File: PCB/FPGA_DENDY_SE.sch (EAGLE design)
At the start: 139 parts, among them CN1 DENDY60PINSLOT, J1 NTSC/PAL, J2 DENDY, Q1 14.318 MHz, Q2 17.734 MHz, U1 EP1C3T100C8N, U10 OPA2134U, U11 SN74LVC2G34DBVR, U12 THS7314DR, U13 74LS373WMSO20, U14 SN74LVC1G125DBVR, U15 74LVC1G04GV, U16 SN74LVC1G3157, U2 EPCS4, U3 SN74LVC8T245, U4 SN74LVC8T245, U5 SN74LVC1G240DBVR, U6 SN74LVC1G240DBVR, U7 SN74LVC1G240DBVR, U8 SN74LVC1G240DBVR, X1 057-010-1

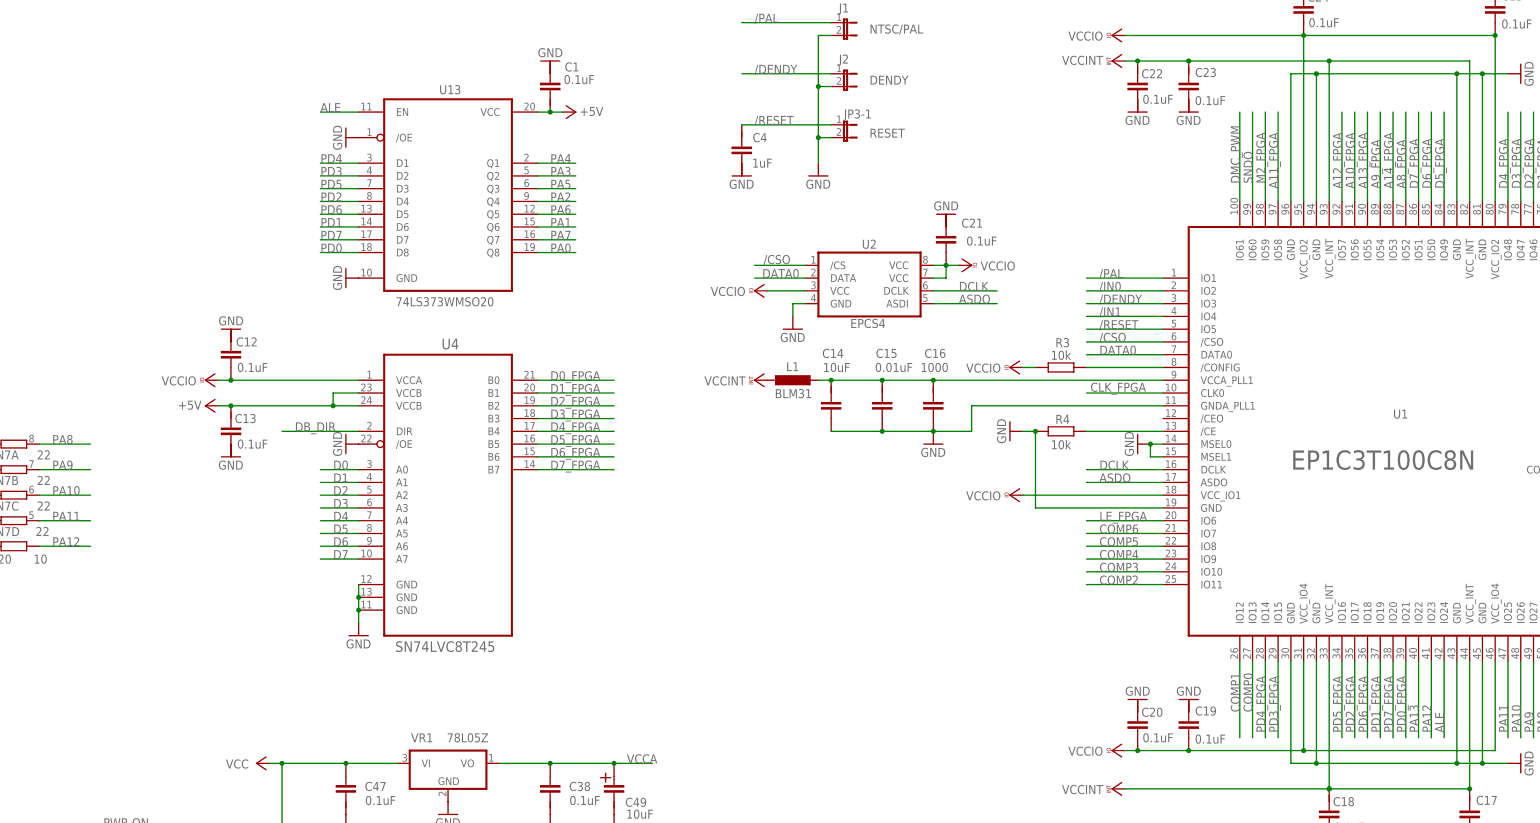
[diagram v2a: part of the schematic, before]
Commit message: Add files via upload
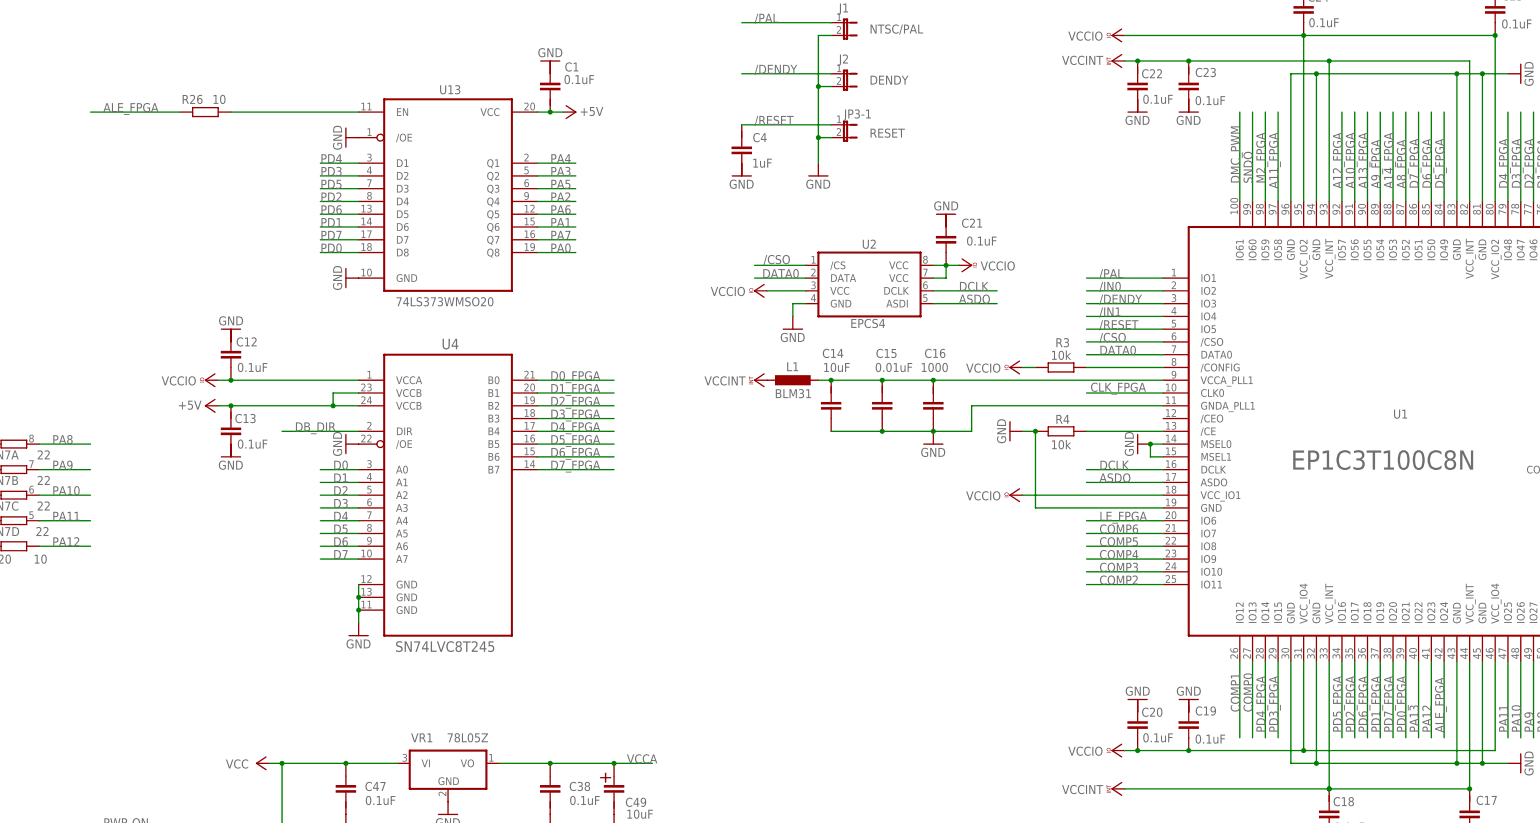
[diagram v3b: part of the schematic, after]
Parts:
- added R26: 10, rcl:R-EU_R0805
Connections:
- removed net ALE: U1.IO24, U13.EN
- new net ALE_FPGA: R26.1, U1.IO24
- new net N$6: R26.2, U13.EN
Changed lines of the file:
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@@
 <setting verticaltext="up"/>
 </settings>
-<grid distance="0.1" unitdist="inch" unit="inch" style="lines" multiple="1" display="no" altdistance="0.01" altunitdist="inch" altunit="inch"/>
+<grid distance="0.1" unitdist="inch" unit="inch" style="lines" multiple="1" display="yes" altdistance="0.01" altunitdist="inch" altunit="inch"/>
 <layers>
-<layer number="1" name="Top" color="4" fill="1" visible="yes" active="no"/>
-<layer number="2" name="Route2" color="16" fill="1" visible="yes" active="no"/>
-<layer number="3" name="Route3" color="17" fill="1" visible="yes" active="no"/>
-<layer number="4" name="Route4" color="18" fill="1" visible="yes" active="no"/>
-<layer number="5" name="Route5" color="19" fill="1" visible="yes" active="no"/>
-<layer number="6" name="Route6" color="25" fill="1" visible="yes" active="no"/>
-<layer number="7" name="Route7" color="26" fill="1" visible="yes" active="no"/>
-<layer number="8" name="Route8" color="27" fill="1" visible="yes" active="no"/>
-<layer number="9" name="Route9" color="28" fill="1" visible="yes" active="no"/>
-<layer number="10" name="Route10" color="29" fill="1" visible="yes" active="no"/>
-<layer number="11" name="Route11" color="30" fill="1" visible="yes" active="no"/>
-<layer number="12" name="Route12" color="20" fill="1" visible="yes" active="no"/>
-<layer number="13" name="Route13" color="21" fill="1" visible="yes" active="no"/>
-<layer number="14" name="Route14" color="22" fill="1" visible="yes" active="no"/>
-<layer number="15" name="Route15" color="23" fill="1" visible="yes" active="no"/>
-<layer number="16" name="Bottom" color="1" fill="1" visible="yes" active="no"/>
-<layer number="17" name="Pads" color="2" fill="1" visible="yes" active="no"/>
-<layer number="18" name="Vias" color="2" fill="1" visible="yes" active="no"/>
-<layer number="19" name="Unrouted" color="6" fill="1" visible="yes" active="no"/>
-<layer number="20" name="Dimension" color="15" fill="1" visible="yes" active="no"/>
-<layer number="21" name="tPlace" color="7" fill="1" visible="yes" active="no"/>
-<layer number="22" name="bPlace" color="7" fill="1" visible="yes" active="no"/>
-<layer number="23" name="tOrigins" color="15" fill="1" visible="yes" active="no"/>
-<layer number="24" name="bOrigins" color="15" fill="1" visible="yes" active="no"/>
-<layer number="25" name="tNames" color="7" fill="1" visible="yes" active="no"/>
-<layer number="26" name="bNames" color="7" fill="1" visible="yes" active="no"/>
-<layer number="27" name="tValues" color="7" fill="1" visible="yes" active="no"/>
-<layer number="28" name="bValues" color="7" fill="1" visible="yes" active="no"/>
+<layer number="1" name="Top" color="4" fill="1" visible="no" active="no"/>
+<layer number="2" name="Route2" color="16" fill="1" visible="no" active="no"/>
+<layer number="3" name="Route3" color="17" fill="1" visible="no" active="no"/>
+<layer number="4" name="Route4" color="18" fill="1" visible="no" active="no"/>
+<layer number="5" name="Route5" color="19" fill="1" visible="no" active="no"/>
+<layer number="6" name="Route6" color="25" fill="1" visible="no" active="no"/>
+<layer number="7" name="Route7" color="26" fill="1" visible="no" active="no"/>
+<layer number="8" name="Route8" color="27" fill="1" visible="no" active="no"/>
+<layer number="9" name="Route9" color="28" fill="1" visible="no" active="no"/>
+<layer number="10" name="Route10" color="29" fill="1" visible="no" active="no"/>
+<layer number="11" name="Route11" color="30" fill="1" visible="no" active="no"/>
+<layer number="12" name="Route12" color="20" fill="1" visible="no" active="no"/>
+<layer number="13" name="Route13" color="21" fill="1" visible="no" active="no"/>
+<layer number="14" name="Route14" color="22" fill="1" visible="no" active="no"/>
+<layer number="15" name="Route15" color="23" fill="1" visible="no" active="no"/>
+<layer number="16" name="Bottom" color="1" fill="1" visible="no" active="no"/>
+<layer number="17" name="Pads" color="2" fill="1" visible="no" active="no"/>
+<layer number="18" name="Vias" color="2" fill="1" visible="no" active="no"/>
+<layer number="19" name="Unrouted" color="6" fill="1" visible="no" active="no"/>
+<layer number="20" name="Dimension" color="15" fill="1" visible="no" active="no"/>
+<layer number="21" name="tPlace" color="7" fill="1" visible="no" active="no"/>
+<layer number="22" name="bPlace" color="7" fill="1" visible="no" active="no"/>
+<layer number="23" name="tOrigins" color="15" fill="1" visible="no" active="no"/>
+<layer number="24" name="bOrigins" color="15" fill="1" visible="no" active="no"/>
+<layer number="25" name="tNames" color="7" fill="1" visible="no" active="no"/>
+<layer number="26" name="bNames" color="7" fill="1" visible="no" active="no"/>
+<layer number="27" name="tValues" color="7" fill="1" visible="no" active="no"/>
+<layer number="28" name="bValues" color="7" fill="1" visible="no" active="no"/>
 <layer number="29" name="tStop" color="7" fill="3" visible="no" active="no"/>
 <layer number="30" name="bStop" color="7" fill="6" visible="no" active="no"/>
@@
 <layer number="35" name="tGlue" color="7" fill="4" visible="no" active="no"/>
 <layer number="36" name="bGlue" color="7" fill="5" visible="no" active="no"/>
-<layer number="37" name="tTest" color="7" fill="1" visible="yes" active="no"/>
-<layer number="38" name="bTest" color="7" fill="1" visible="yes" active="no"/>
+<layer number="37" name="tTest" color="7" fill="1" visible="no" active="no"/>
+<layer number="38" name="bTest" color="7" fill="1" visible="no" active="no"/>
 <layer number="39" name="tKeepout" color="4" fill="11" visible="no" active="no"/>
 <layer number="40" name="bKeepout" color="1" fill="11" visible="no" active="no"/>
@@
 <layer number="44" name="Drills" color="7" fill="1" visible="no" active="no"/>
 <layer number="45" name="Holes" color="7" fill="1" visible="no" active="no"/>
-<layer number="46" name="Milling" color="3" fill="1" visible="yes" active="no"/>
-<layer number="47" name="Measures" color="7" fill="1" visible="yes" active="no"/>
-<layer number="48" name="Document" color="7" fill="1" visible="yes" active="no"/>
-<layer number="49" name="Reference" color="7" fill="1" visible="yes" active="no"/>
-<layer number="50" name="dxf" color="7" fill="1" visible="yes" active="no"/>
-<layer number="51" name="tDocu" color="7" fill="1" visible="yes" active="no"/>
-<layer number="52" name="bDocu" color="7" fill="1" visible="yes" active="no"/>
-<layer number="56" name="wert" color="7" fill="1" visible="yes" active="no"/>
+<layer number="46" name="Milling" color="3" fill="1" visible="no" active="no"/>
+<layer number="47" name="Measures" color="7" fill="1" visible="no" active="no"/>
+<layer number="48" name="Document" color="7" fill="1" visible="no" active="no"/>
+<layer number="49" name="Reference" color="7" fill="1" visible="no" active="no"/>
+<layer number="50" name="dxf" color="7" fill="1" visible="no" active="no"/>
+<layer number="51" name="tDocu" color="7" fill="1" visible="no" active="no"/>
+<layer number="52" name="bDocu" color="7" fill="1" visible="no" active="no"/>
+<layer number="56" name="wert" color="7" fill="1" visible="no" active="no"/>
 <layer number="88" name="SimResults" color="9" fill="1" visible="yes" active="yes"/>
 <layer number="89" name="SimProbes" color="9" fill="1" visible="yes" active="yes"/>
@@
 <part name="GND81" library="supply1" library_urn="urn:adsk.eagle:library:371" deviceset="GND" device=""/>
 <part name="VCC15" library="supply1" library_urn="urn:adsk.eagle:library:371" deviceset="VCCIO" device=""/>
+<part name="R26" library="rcl" library_urn="urn:adsk.eagle:library:334" deviceset="R-EU_" device="R0805" package3d_urn="urn:adsk.eagle:package:23553/2" value="10"/>
 </parts>
 <sheets>
@@
 <attribute name="VALUE" x="29.718" y="158.242" size="1.778" layer="96" rot="MR180"/>
 </instance>
+<instance part="R26" gate="G$1" x="-236.22" y="60.96" smashed="yes">
+<attribute name="NAME" x="-236.648" y="64.3626" size="1.778" layer="95" rot="R180"/>
+<attribute name="VALUE" x="-232.068" y="64.368" size="1.778" layer="96" rot="R180"/>
+</instance>
 </instances>
 <busses>
@@
 </segment>
 </net>
-<net name="ALE" class="0">
-<segment>
-<wire x1="10.16" y1="-48.26" x2="10.16" y2="-63.5" width="0.1524" layer="91"/>
-<label x="10.16" y="-62.484" size="1.778" layer="95" rot="R90"/>
-<pinref part="U1" gate="G$1" pin="IO24"/>
-</segment>
-<segment>
-<wire x1="-205.74" y1="60.96" x2="-213.36" y2="60.96" width="0.1524" layer="91"/>
-<label x="-213.36" y="60.96" size="1.778" layer="95"/>
-<pinref part="U13" gate="G$1" pin="EN"/>
-</segment>
-</net>
 <net name="N$17" class="0">
 <segment>
@@
 </segment>
 </net>
+<net name="ALE_FPGA" class="0">
+<segment>
+<wire x1="10.16" y1="-48.26" x2="10.16" y2="-63.5" width="0.1524" layer="91"/>
+<label x="10.16" y="-62.484" size="1.778" layer="95" rot="R90"/>
+<pinref part="U1" gate="G$1" pin="IO24"/>
+</segment>
+<segment>
+<pinref part="R26" gate="G$1" pin="1"/>
+<wire x1="-241.3" y1="60.96" x2="-259.08" y2="60.96" width="0.1524" layer="91"/>
+<label x="-256.54" y="60.96" size="1.778" layer="95"/>
+</segment>
+</net>
+<net name="N$6" class="0">
+<segment>
+<pinref part="U13" gate="G$1" pin="EN"/>
+<pinref part="R26" gate="G$1" pin="2"/>
+<wire x1="-205.74" y1="60.96" x2="-231.14" y2="60.96" width="0.1524" layer="91"/>
+</segment>
+</net>
